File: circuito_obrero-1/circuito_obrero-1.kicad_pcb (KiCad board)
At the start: 2 copper layers, 40 parts, among them J1 Conn_01x03_Pin, J10 Conn_01x05, J2 Conn_01x03_Pin, J3 Conn_01x03_Pin, J4 Conn_01x03_Pin, J5 Conn_01x03_Pin, J6 Conn_01x03_Pin, J7 Conn_01x03_Pin, J8 Conn_01x03_Pin, J9 Conn_01x05, U1 74HC165, U2 74HC165, U3 74HC165

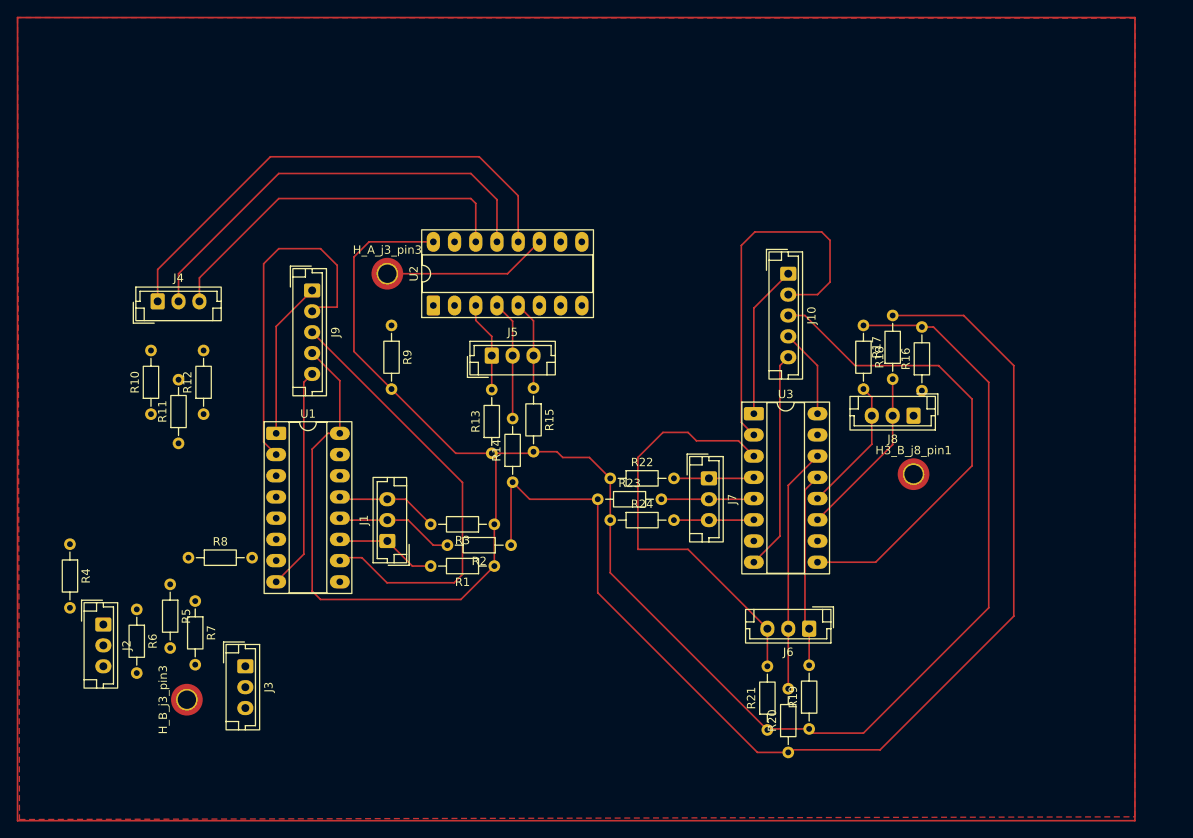
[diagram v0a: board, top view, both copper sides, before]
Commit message: pre añadir lagrimas
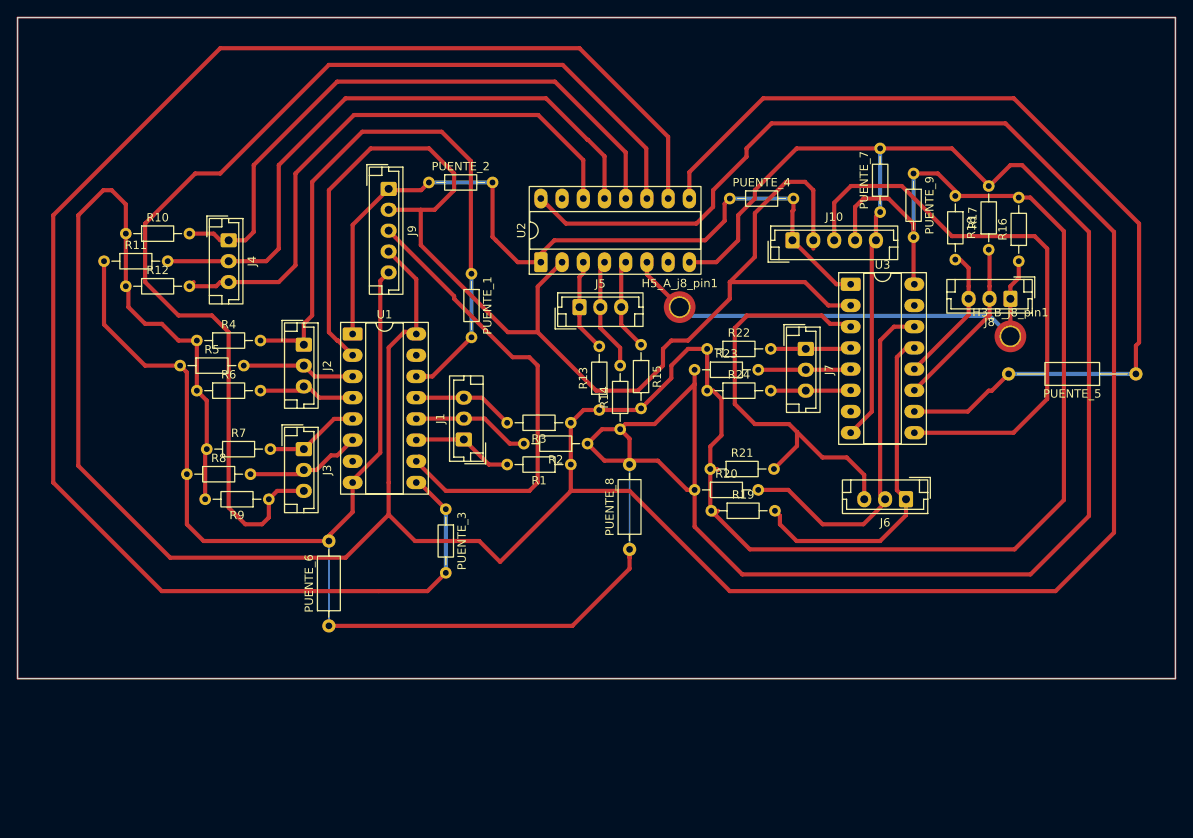
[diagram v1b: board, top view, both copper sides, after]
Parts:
- removed H_A_j3_pin3, H_B_j3_pin3: MountingHole_Pad, MountingHole:MountingHole_2.2mm_M2_DIN965_Pad_TopOnly
- added H5_A_j8_pin1: MountingHole_Pad, MountingHole:MountingHole_2.2mm_M2_DIN965_Pad_TopOnly, F.Cu at (148.0, 68.0)
- added PUENTE_1: 0k, Resistor_THT:R_Axial_DIN0204_L3.6mm_D1.6mm_P7.62mm_Horizontal, F.Cu at (123.1, 64.0)
- added PUENTE_2: 0k, Resistor_THT:R_Axial_DIN0204_L3.6mm_D1.6mm_P7.62mm_Horizontal, F.Cu at (118.0, 53.1)
- added PUENTE_3: 0k, Resistor_THT:R_Axial_DIN0204_L3.6mm_D1.6mm_P7.62mm_Horizontal, F.Cu at (120.0, 92.2)
- added PUENTE_4: 0k, Resistor_THT:R_Axial_DIN0204_L3.6mm_D1.6mm_P7.62mm_Horizontal, F.Cu at (154.0, 55.0)
- added PUENTE_5: 0k, Resistor_THT:R_Axial_DIN0207_L6.3mm_D2.5mm_P15.24mm_Horizontal, F.Cu at (202.6, 76.0)
- added PUENTE_6: 0k, Resistor_THT:R_Axial_DIN0207_L6.3mm_D2.5mm_P10.16mm_Horizontal, F.Cu at (106.0, 106.2)
- added PUENTE_7: 0k, Resistor_THT:R_Axial_DIN0204_L3.6mm_D1.6mm_P7.62mm_Horizontal, F.Cu at (172.0, 56.6)
- added PUENTE_8: 0k, Resistor_THT:R_Axial_DIN0207_L6.3mm_D2.5mm_P10.16mm_Horizontal, F.Cu at (142.0, 97.0)
- added PUENTE_9: 0k, Resistor_THT:R_Axial_DIN0204_L3.6mm_D1.6mm_P7.62mm_Horizontal, F.Cu at (176.0, 52.0)
- moved J2 41.2 mm to (103.0, 72.5)
- moved R20 33.4 mm to (149.8, 89.9), turned to 0 degrees
- moved R21 32.0 mm to (151.7, 87.4), turned to 0 degrees
- moved R4 28.7 mm to (90.2, 72.0), turned to 0 degrees
- moved R19 28.6 mm to (151.8, 92.4), turned to 0 degrees
- moved R6 27.2 mm to (90.2, 78.0), turned to 0 degrees
- moved J3 26.9 mm to (103.0, 85.0)
- moved R5 26.2 mm to (88.2, 75.0), turned to 0 degrees
- moved R9 25.5 mm to (98.8, 91.0), turned to 180 degrees
- moved R11 23.6 mm to (79.1, 62.5), turned to 0 degrees
- moved R10 21.8 mm to (81.7, 59.2), turned to 0 degrees
- moved H3_B_j8_pin1 20.2 mm to (187.6, 71.5)
- moved J6 19.4 mm to (175.1, 91.0)
- moved J7 19.4 mm to (163.1, 73.0)
- moved R16 19.4 mm to (188.6, 62.5)
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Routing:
- net VCC: track 254.9 -> 556.6 mm
- net GND: track 194.2 -> 392.7 mm
- net Net-(U1-Q7): track 0.00 -> 191.5 mm
- net Net-(U2-Q7): track 0.00 -> 113.4 mm
- net Net-(J3-Pin_3): track 19.8 -> 131.3 mm
- net Net-(J2-Pin_1): track 0.00 -> 79.2 mm
- net Net-(J10-Pin_2): track 87.7 -> 157.7 mm
- net Net-(J8-Pin_1): track 0.00 -> 57.5 mm
- net Net-(J10-Pin_1): track 37.4 -> 94.7 mm
- net Net-(J4-Pin_3): track 44.7 -> 69.6 mm
- net Net-(J4-Pin_2): track 52.8 -> 74.2 mm
- net Net-(J6-Pin_1): track 23.3 -> 41.0 mm
- net Net-(J4-Pin_1): track 60.0 -> 74.2 mm
- net Net-(J3-Pin_2): track 0.00 -> 13.9 mm
- net Net-(J2-Pin_2): track 0.00 -> 13.6 mm
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- removed copper zone on F.Cu, net GND
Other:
- board outline added: 138.6 x 79.1 mm
